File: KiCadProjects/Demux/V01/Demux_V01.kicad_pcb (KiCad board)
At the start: 2 copper layers, 90 x 100 mm, 40 parts, among them J1 alimentacao analogica, J12 +9Vmux, J13 +5Vmux, J14 +3.3Vmux, J15 -9Vmux, J16 -5Vmux, J17 GNDmux, J18 Conn_01x03, J19 Conn_01x06, J2 sinais analogicos, J20 Conn_01x06, J21 Conn_01x06, J22 Conn_01x06, J23 Conn_01x06, J24 Conn_01x06, J25 Conn_01x06, J26 Conn_01x06, J27 Conn_01x06, J28 Conn_01x06, J29 Conn_01x06, J3 comunicacao / sinais digitais, J30 Conn_01x06, J31 Conn_01x06, J32 Conn_01x06, J33 Conn_01x06, J34 Conn_01x06, J4 Conn_01x02, J5 Conn_01x02, J6 Conn_01x02, U1A1 74HC4051, U1B1 74HC4051, U2 BluePill_STM32F103C, U2A2 74HC4051, U2B2 74HC4051, U3A3 74HC4051, U3B3 74HC4051, U4A4 74HC4051, U4B4 74HC4051, U5A1 74HC4051, U5B1 74HC4051

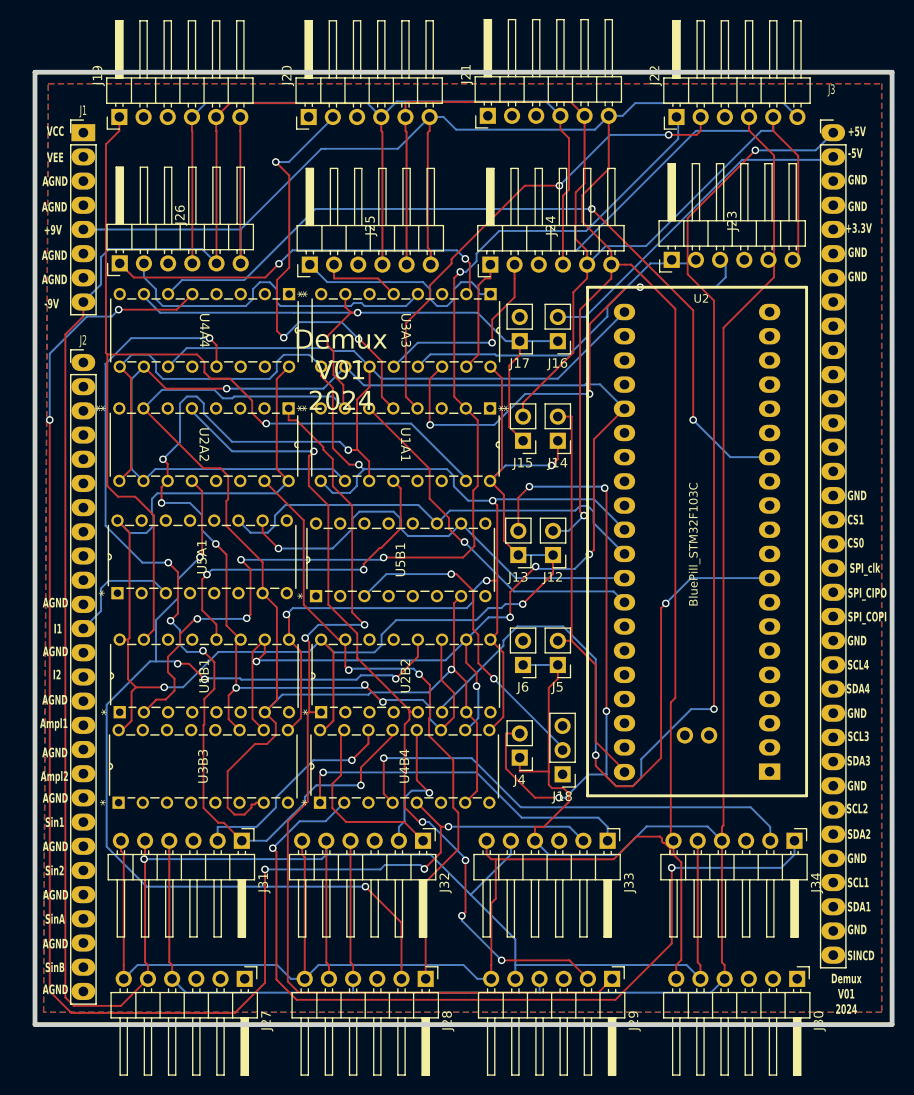
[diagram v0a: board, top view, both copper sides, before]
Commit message: placa em producao
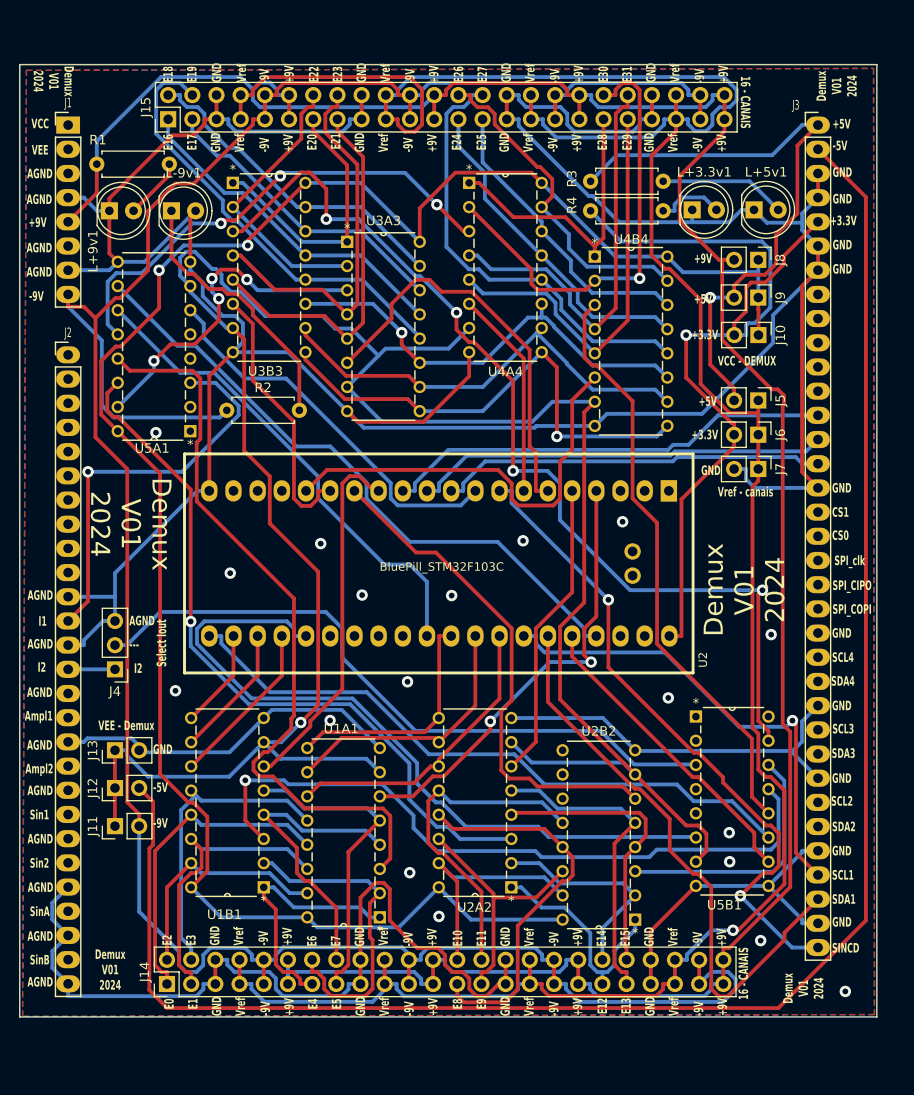
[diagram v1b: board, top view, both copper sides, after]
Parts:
- removed J16: -5Vmux, Connector_PinHeader_2.54mm:PinHeader_1x02_P2.54mm_Vertical
- removed J17: GNDmux, Connector_PinHeader_2.54mm:PinHeader_1x02_P2.54mm_Vertical
- removed J18: Conn_01x03, Connector_PinHeader_2.54mm:PinHeader_1x03_P2.54mm_Vertical
- removed J19, J20, J21, J22, J23, J24, J25, J26, J27, J28, J29, J30, J31, J32, J33, J34: Conn_01x06, Connector_PinHeader_2.54mm:PinHeader_1x06_P2.54mm_Horizontal
- added J10: +3.3Vmux, Connector_PinHeader_2.54mm:PinHeader_1x02_P2.54mm_Vertical, F.Cu at (177.6, 78.4)
- added J11: -9Vmux, Connector_PinHeader_2.54mm:PinHeader_1x02_P2.54mm_Vertical, F.Cu at (110.0, 130.0)
- added J7: Conn_01x02, Connector_PinHeader_2.54mm:PinHeader_1x02_P2.54mm_Vertical, F.Cu at (177.6, 92.5)
- added J8: +9Vmux, Connector_PinHeader_2.54mm:PinHeader_1x02_P2.54mm_Vertical, F.Cu at (177.6, 70.5)
- added J9: +5Vmux, Connector_PinHeader_2.54mm:PinHeader_1x02_P2.54mm_Vertical, F.Cu at (177.6, 74.5)
- added L+3.3v1: LED Yelow, LED_THT:LED_D5.0mm, F.Cu at (170.6, 65.2)
- added L+5v1: LED Green, LED_THT:LED_D5.0mm, F.Cu at (177.1, 65.2)
- added L+9v1: LED Blue, LED_THT:LED_D5.0mm, F.Cu at (109.4, 65.3)
- added L-9v1: LED Red, LED_THT:LED_D5.0mm, F.Cu at (115.9, 65.3)
- added R1: 1.5k, Resistor_THT:R_Axial_DIN0207_L6.3mm_D2.5mm_P7.62mm_Horizontal, F.Cu at (108.1, 60.5)
- added R2: 1.5k, Resistor_THT:R_Axial_DIN0207_L6.3mm_D2.5mm_P7.62mm_Horizontal, F.Cu at (121.7, 86.3)
- added R3: 470, Resistor_THT:R_Axial_DIN0207_L6.3mm_D2.5mm_P7.62mm_Horizontal, F.Cu at (159.9, 62.2)
- added R4: 510, Resistor_THT:R_Axial_DIN0207_L6.3mm_D2.5mm_P7.62mm_Horizontal, F.Cu at (159.9, 65.3)
- J12: value +9Vmux -> -5Vmux
- J13: value +5Vmux -> GNDmux
- J14: value +3.3Vmux -> conectorEletrodos; footprint Connector_PinHeader_2.54mm:PinHeader_1x02_P2.54mm_Vertical -> Connector_PinHeader_2.54mm:PinHeader_2x24_P2.54mm_Vertical
- J15: value -9Vmux -> conectorEletrodos; footprint Connector_PinHeader_2.54mm:PinHeader_1x02_P2.54mm_Vertical -> Connector_PinHeader_2.54mm:PinHeader_2x24_P2.54mm_Vertical
- J4: value Conn_01x02 -> Conn_01x03; footprint Connector_PinHeader_2.54mm:PinHeader_1x02_P2.54mm_Vertical -> Connector_PinHeader_2.54mm:PinHeader_1x03_P2.54mm_Vertical
- moved J14 70.3 mm to (115.5, 146.5), turned to 90 degrees
- moved J12 52.1 mm to (110.0, 126.0), turned to 90 degrees
- moved J15 50.3 mm to (115.6, 55.7), turned to 90 degrees
- moved U5B1 48.3 mm to (178.6, 136.2), turned to 0 degrees
- moved J13 47.1 mm to (110.0, 122.0), turned to 90 degrees
- moved U4A4 44.3 mm to (154.8, 80.2), turned to 0 degrees
- moved J4 43.5 mm to (110.0, 113.5)
- moved U2A2 41.8 mm to (144.0, 118.6), turned to 180 degrees
- moved U3B3 39.7 mm to (130.0, 80.2), turned to 0 degrees
- moved U4B4 37.0 mm to (168.0, 87.9), turned to 0 degrees
- moved J5 34.9 mm to (177.6, 85.3), turned to -90 degrees
- moved J6 34.6 mm to (177.6, 88.9), turned to -90 degrees
- moved U5A1 32.5 mm to (110.3, 70.7), turned to 180 degrees
- moved U2 31.3 mm to (168.1, 94.8), turned to -90 degrees
- moved U1A1 28.1 mm to (130.2, 121.8), turned to 180 degrees
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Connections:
- J12 pad 1: VCC_DEMUX -> VEE_DEMUX
- J12 pad 2: +9V -> -5V
- J13 pad 1: VCC_DEMUX -> VEE_DEMUX
- J13 pad 2: +5V -> Earth
- J14 pad 1: VCC_DEMUX -> E0
- J14 pad 2: +3.3V -> E1
- J15 pad 1: VEE_DEMUX -> E16
- J15 pad 2: -9V -> E17
- J3 pad 13: unconnected-(J3-Pin_13-Pad13) -> SINC_C
- J3 pad 14: unconnected-(J3-Pin_14-Pad14) -> SINC_B
- J3 pad 15: unconnected-(J3-Pin_15-Pad15) -> SINC_A
- J4 pad 1: Vref -> I2
- J4 pad 2: +5V -> In_B
- J5 pad 2: +3.3V -> +5V
- J6 pad 2: Earth -> +3.3V
- U1A1 pad 10: S1 -> A_S1
- U1A1 pad 11: S0 -> A_S0
- U1A1 pad 3: DEMUX1 -> DEMUXA1
- U1A1 pad 9: S2 -> A_S2
- U1B1 pad 10: S1 -> B_S1
- U1B1 pad 11: S0 -> B_S0
- U1B1 pad 3: DEMUX1B -> DEMUXB1
- U1B1 pad 9: S2 -> B_S2
- U2 pad 10: unconnected-(U2-PA5_SCK1-Pad10) -> SINC_A
- U2 pad 11: unconnected-(U2-PA6_MISO1-Pad11) -> SINC_B
- U2 pad 12: unconnected-(U2-PA7_MOSI1-Pad12) -> SINC_C
- U2 pad 14: Enable_A4 -> Enable_B2
- U2 pad 15: unconnected-(U2-PB10_SCL2-Pad15) -> Enable_B3
- U2 pad 16: unconnected-(U2-PB11_SDA2-Pad16) -> Enable_B4
- U2 pad 21: S0 -> B_S3
- U2 pad 22: unconnected-(U2-PB13_SCK2-Pad22) -> B_S2
- U2 pad 23: unconnected-(U2-PB14_MISO2-Pad23) -> B_S1
- U2 pad 24: unconnected-(U2-PB15_MOSI2-Pad24) -> B_S0
- U2 pad 25: S1 -> Enable_B
- U2 pad 30: S2 -> A_S3
- U2 pad 31: S3 -> A_S2
- U2 pad 32: S4 -> A_S1
- U2 pad 33: Enable_A1 -> A_S0
- U2 pad 34: unconnected-(U2-PB6_SCL1-Pad34) -> SCL1
- U2 pad 35: unconnected-(U2-PB7_SDA1-Pad35) -> SDA1
- U2 pad 36: Enable_A2 -> B_S4
- U2 pad 37: Enable_A3 -> A_S4
- U2 pad 4: unconnected-(U2-PC15-Pad4) -> Enable_A1
- U2 pad 5: Enable_B4 -> Enable_A2
- U2 pad 6: Enable_B3 -> Enable_A3
- U2 pad 7: unconnected-(U2-PA2_TX2-Pad7) -> Enable_A4
- U2 pad 8: unconnected-(U2-PA3_RX2-Pad8) -> SINCD
- U2 pad 9: Enable_B2 -> Enable_A
- U2A2 pad 10: S1 -> A_S1
- U2A2 pad 11: S0 -> A_S0
- U2A2 pad 3: DEMUX2A -> DEMUXA2
- U2A2 pad 9: S2 -> A_S2
- U2B2 pad 10: S1 -> SB1
- U2B2 pad 11: S0 -> SB0
- U2B2 pad 3: DEMUX2B -> DEMUXB2
- U2B2 pad 9: S2 -> SB2
- U3A3 pad 3: DEMUX3A -> DEMUXA3
- U3B3 pad 3: DEMUX3B -> DEMUXB3
- U4A4 pad 3: DEMUX4A -> DEMUXA4
- U4B4 pad 3: DEMUX4B -> DEMUXB4
- U5A1 pad 10: S4 -> A_S4
- U5A1 pad 11: S3 -> A_S3
- U5A1 pad 6: Earth -> Enable_A
- U5B1 pad 10: S4 -> B_S4
- U5B1 pad 11: S3 -> B_S3
- U5B1 pad 6: Earth -> Enable_B
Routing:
- net Earth: track 0.00 -> 527.7 mm, vias 0 -> 18
- net -5V: track 35.9 -> 184.9 mm
- net S1: track 171.6 -> 47.1 mm, vias 6 -> 0
- net E29: track 162.7 -> 43.1 mm, vias 5 -> 0
- net S0: track 164.8 -> 47.4 mm, vias 7 -> 1
- net DEMUXB3: track 0.00 -> 103.5 mm, vias 0 -> 4
- net S2: track 152.7 -> 52.0 mm, vias 4 -> 1
- net -9V: track 373.3 -> 277.8 mm, vias 1 -> 0
- net +9V: track 353.6 -> 259.7 mm, vias 1 -> 0
- net +5V: track 149.3 -> 63.7 mm, vias 6 -> 1
- net E12: track 106.9 -> 23.7 mm, vias 2 -> 0
- net Vref: track 354.1 -> 273.8 mm, vias 0 -> 1
- net E11: track 115.0 -> 35.2 mm, vias 5 -> 0
- net DEMUXA1: track 0.00 -> 79.5 mm
- net E2: track 103.8 -> 24.7 mm, vias 1 -> 0
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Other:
- board text added: "---"
- board text added: "16 - CANAIS"
- board text added: "E0"
- board text added: "E1"
- board text added: "E10"
- board text added: "E11"
- board text added: "E12"
- board text added: "E13"
- board text added: "E14"
- board text added: "E15"
- board text added: "E16"
- board text added: "E17"
- board text added: "E18"
- board text added: "E19"
- board text added: "E2"
- board text added: "E20"
- board text added: "E21"
- board text added: "E22"
- board text added: "E23"
- board text added: "E24"
- board text added: "E25"
- board text added: "E26"
- board text added: "E27"
- board text added: "E28"
- board text added: "E29"
- board text added: "E3"
- board text added: "E30"
- board text added: "E31"
- board text added: "E4"
- board text added: "E5"
- board text added: "E6"
- board text added: "E7"
- board text added: "E8"
- board text added: "E9"
- board text added: "Select Iout"
- board text added: "VCC - DEMUX"
- board text added: "VEE - Demux"
- board text added: "Vref"
- board text added: "Vref - canais"
